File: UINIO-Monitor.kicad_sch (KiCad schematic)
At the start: 22 parts

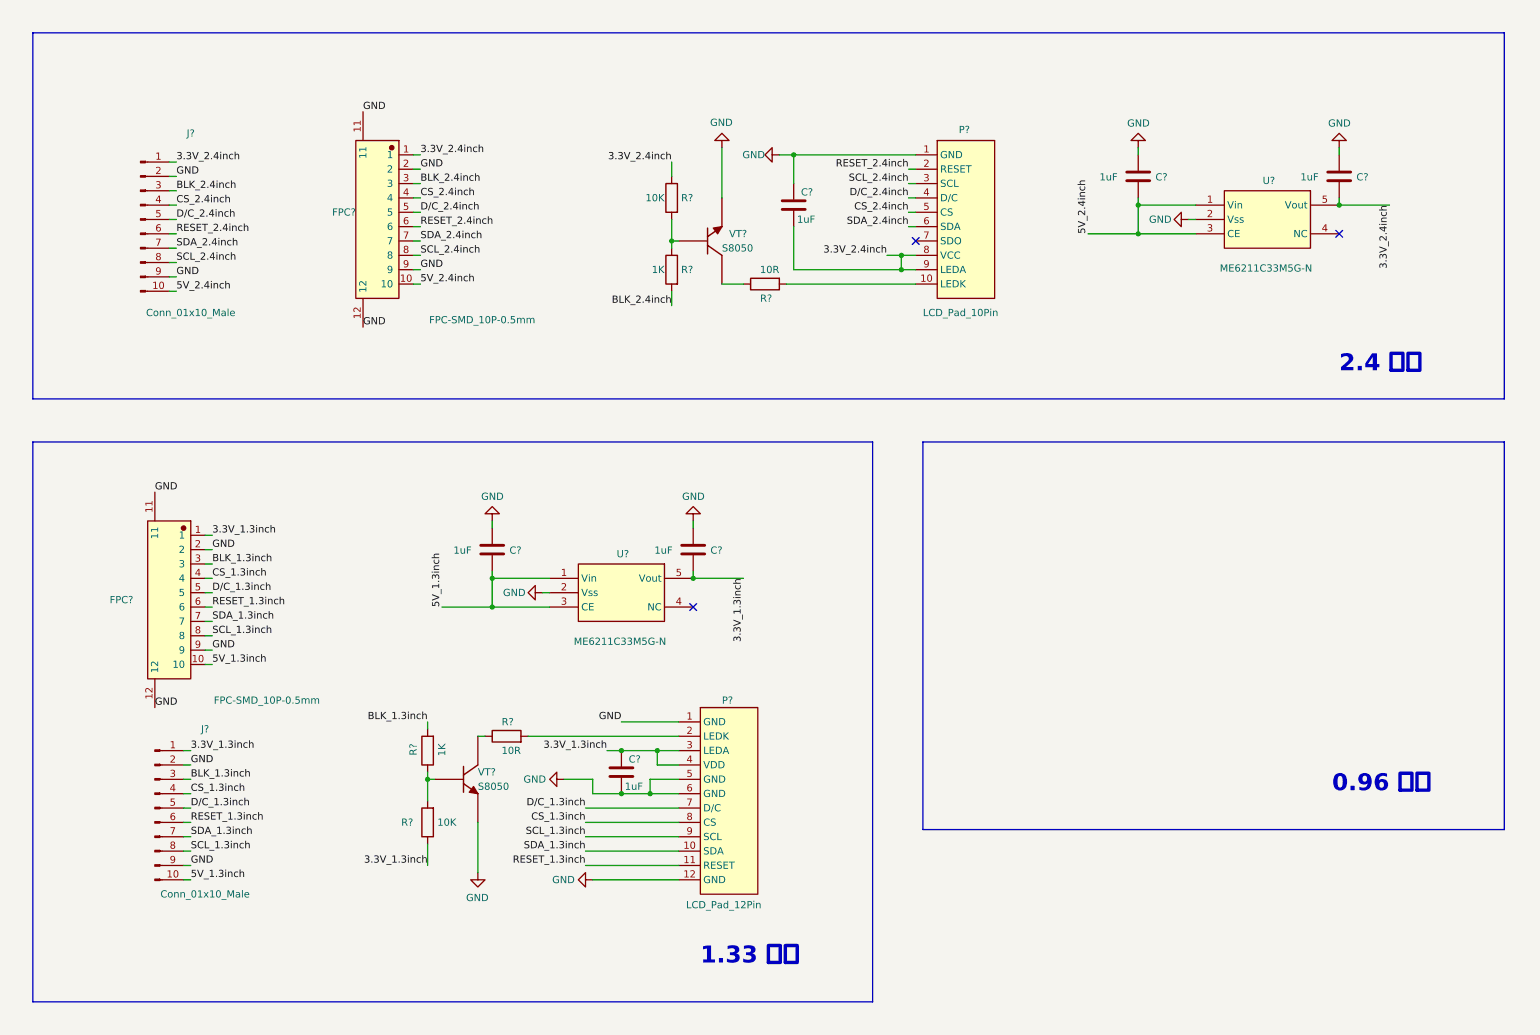
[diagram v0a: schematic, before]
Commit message: Complete schematic drawing.
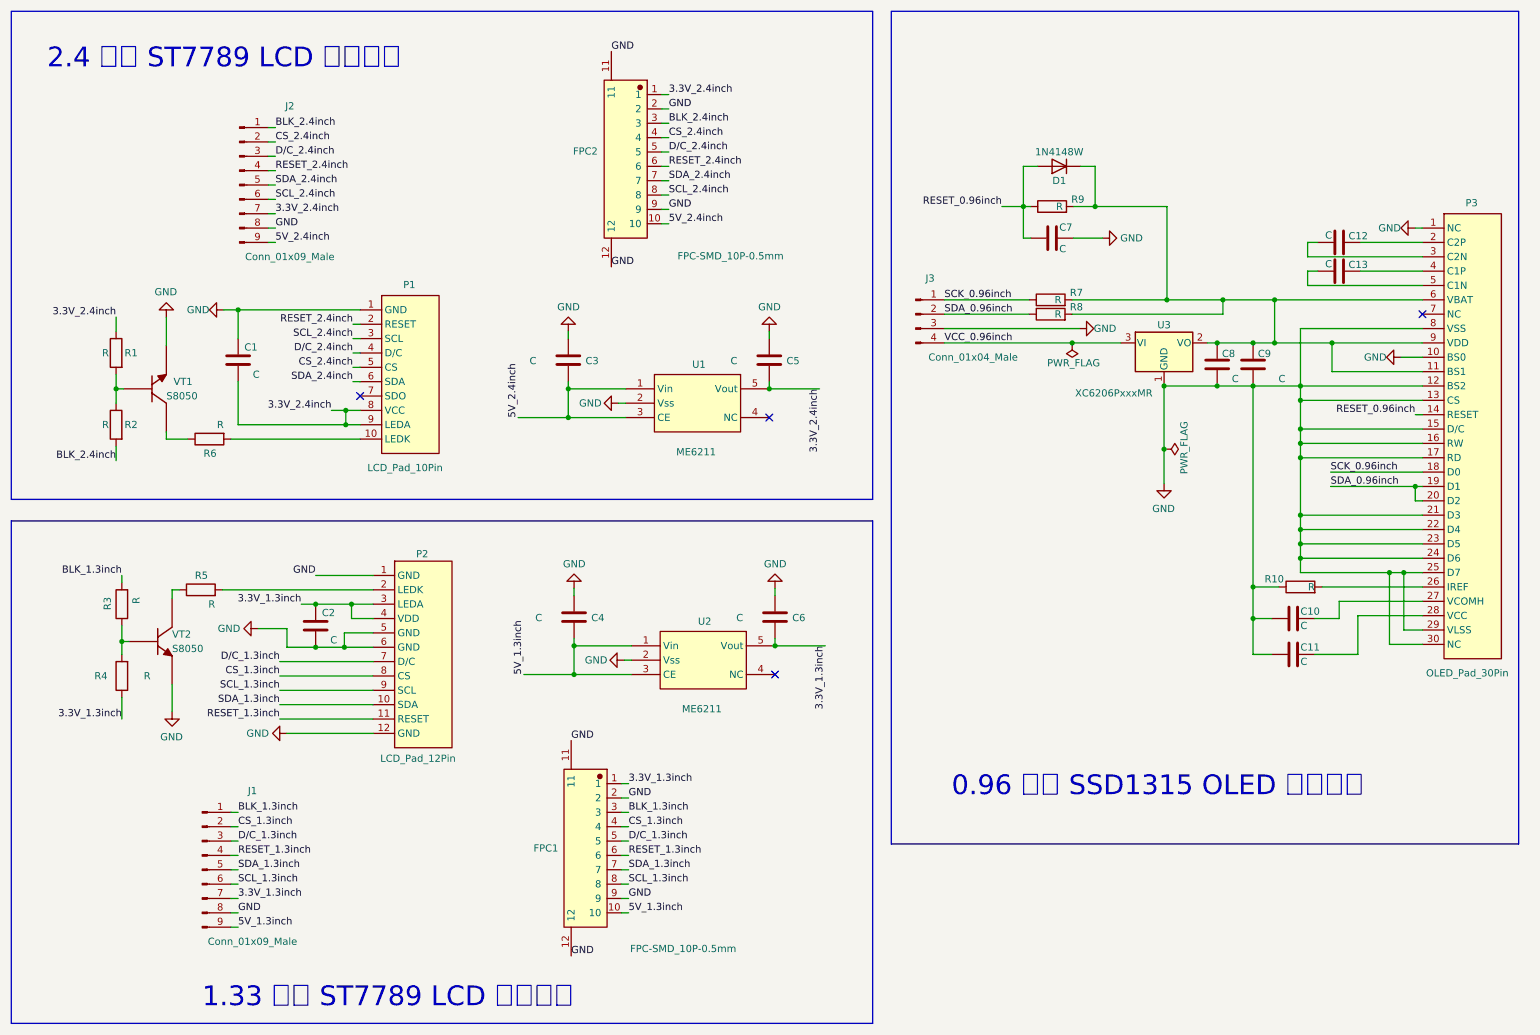
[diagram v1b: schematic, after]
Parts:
- removed J? (x2): Conn_01x10_Male, symbol Connector:Conn_01x10_Male
- added C10, C11, C12, C13, C8, C9: C, Capacitor_SMD:C_0402_1005Metric, symbol Device:C
- added C7: C, Capacitor_SMD:C_0603_1608Metric, symbol Device:C
- added D1: 1N4148W, Diode_SMD:D_SOD-123, symbol Diode:1N4148W
- added J1, J2: Conn_01x09_Male, Connector_PinHeader_2.54mm:PinHeader_1x09_P2.54mm_Vertical, symbol Connector:Conn_01x09_Male
- added J3: Conn_01x04_Male, Connector_PinHeader_2.54mm:PinHeader_1x04_P2.54mm_Vertical, symbol Connector:Conn_01x04_Male
- added P3: OLED_Pad_30Pin, Uinio:OLED_Pad_30Pin, symbol Uinio:OLED_Pad_30Pin
- added R10, R7, R8, R9: R, Resistor_SMD:R_0402_1005Metric, symbol Device:R
- added U3: XC6206PxxxMR, Package_TO_SOT_SMD:SOT-23-3, symbol Regulator_Linear:XC6206PxxxMR
- C1, C2, C3, C4, C5, C6: renamed from C?; value 1uF -> C; footprint Capacitor_SMD:C_0402_1005Metric -> Capacitor_SMD:C_0603_1608Metric
- P1: renamed from P?; footprint (none) -> Uinio:LCD_Pad_10Pin
- P2: renamed from P?; footprint Uinio:ST7789-FPC-PAD -> Uinio:LCD_Pad_12Pin
- R1, R4: renamed from R?; value 10K -> R; footprint (none) -> Resistor_SMD:R_0603_1608Metric
- R2, R3: renamed from R?; value 1K -> R; footprint (none) -> Resistor_SMD:R_0603_1608Metric
- R5, R6: renamed from R?; value 10R -> R; footprint (none) -> Resistor_SMD:R_0603_1608Metric
- U1, U2: renamed from U?; value ME6211C33M5G-N -> ME6211
- gave numbers to parts that had none: 4
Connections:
- net 3.3V_1.3inch: now also J1.7 (Pin_7)
- net 3.3V_2.4inch: now also J2.7 (Pin_7)
- net 5V_1.3inch: now also J1.9 (Pin_9)
- net 5V_2.4inch: now also J2.9 (Pin_9)
- net BLK_1.3inch: now also J1.1 (Pin_1)
- net BLK_2.4inch: now also J2.1 (Pin_1)
- net CS_1.3inch: now also J1.2 (Pin_2)
- net CS_2.4inch: now also J2.2 (Pin_2)
- net D/C_1.3inch: now also J1.3 (Pin_3)
- net D/C_2.4inch: now also J2.3 (Pin_3)
- net GND: now also C10.2, C11.2, C7.1, C8.1, C9.1, J1.8 (Pin_8), J2.8 (Pin_8), J3.3 (Pin_3), P3.1 (NC), P3.10 (BS0), P3.12 (BS2), P3.13 (CS), P3.15 (D/C), P3.16 (RW), P3.17 (RD), P3.21 (D3), P3.22 (D4), P3.23 (D5), P3.24 (D6), P3.25 (D7), P3.29 (VLSS), P3.30 (NC), P3.8 (VSS), R10.1, U3.1 (GND)
- net RESET_1.3inch: now also J1.4 (Pin_4)
- net RESET_2.4inch: now also J2.4 (Pin_4)
- net SCL_1.3inch: now also J1.6 (Pin_6)
- net SCL_2.4inch: now also J2.6 (Pin_6)
- net SDA_1.3inch: now also J1.5 (Pin_5)
- net SDA_2.4inch: now also J2.5 (Pin_5)
- new net: C8.2, C9.2, D1.1 (K), P3.11 (BS1), P3.6 (VBAT), P3.9 (VDD), R7.2, R8.2, R9.2, U3.2 (VO)
- new net: C13.1, P3.5 (C1N)
- new net: C13.2, P3.4 (C1P)
- new net: C12.1, P3.3 (C2N)
- new net: C12.2, P3.2 (C2P)
- new net: P3.26 (IREF), R10.2
- new net: C10.1, P3.27 (VCOMH)
- new net: C11.1, P3.28 (VCC)
- new net RESET_0.96inch: C7.2, D1.2 (A), P3.14 (RESET), R9.1
- new net SCK_0.96inch: J3.1 (Pin_1), P3.18 (D0), R7.1
- new net SDA_0.96inch: J3.2 (Pin_2), P3.19 (D1), P3.20 (D2), R8.1
- new net VCC_0.96inch: J3.4 (Pin_4), U3.3 (VI)
- no-connect marks 3 -> 4
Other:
- note added: "0.96 英寸 SSD1315 OLED 屏幕基板"
- note added: "1.33 英寸 ST7789 LCD 屏幕基板"
- note added: "2.4 英寸 ST7789 LCD 屏幕基板"
- note removed: "0.96 英寸"
- note removed: "1.33 英寸"
- note removed: "2.4 英寸"
- moved on the sheet: C1, C2, C3, C4, C5, C6, FPC1, FPC2, P1, P2, R1, R2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
